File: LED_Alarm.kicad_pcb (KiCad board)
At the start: 2 copper layers, 48.3 x 82.8 mm, 84 parts, among them P101 CONN_01X06, Q301 Q_NPN_BCE, Q401 FDMA410NZT, Q402 FDMA410NZT, Q403 FDMA410NZT, Q501 FDMA410NZT, Q502 FDMA410NZT, Q503 FDMA410NZT, Q601 FDMA410NZT, Q602 FDMA410NZT, Q603 FDMA410NZT, Q701 FDMA410NZT, Q702 FDMA410NZT, Q703 FDMA410NZT, Q801 FDMA410NZT, Q802 FDMA410NZT, Q803 FDMA410NZT, U101 H11AA11, U102 ESP-12, U103 PCA9685PW, U201 MOC3020M, U202 TRIAC, U901 XC9263

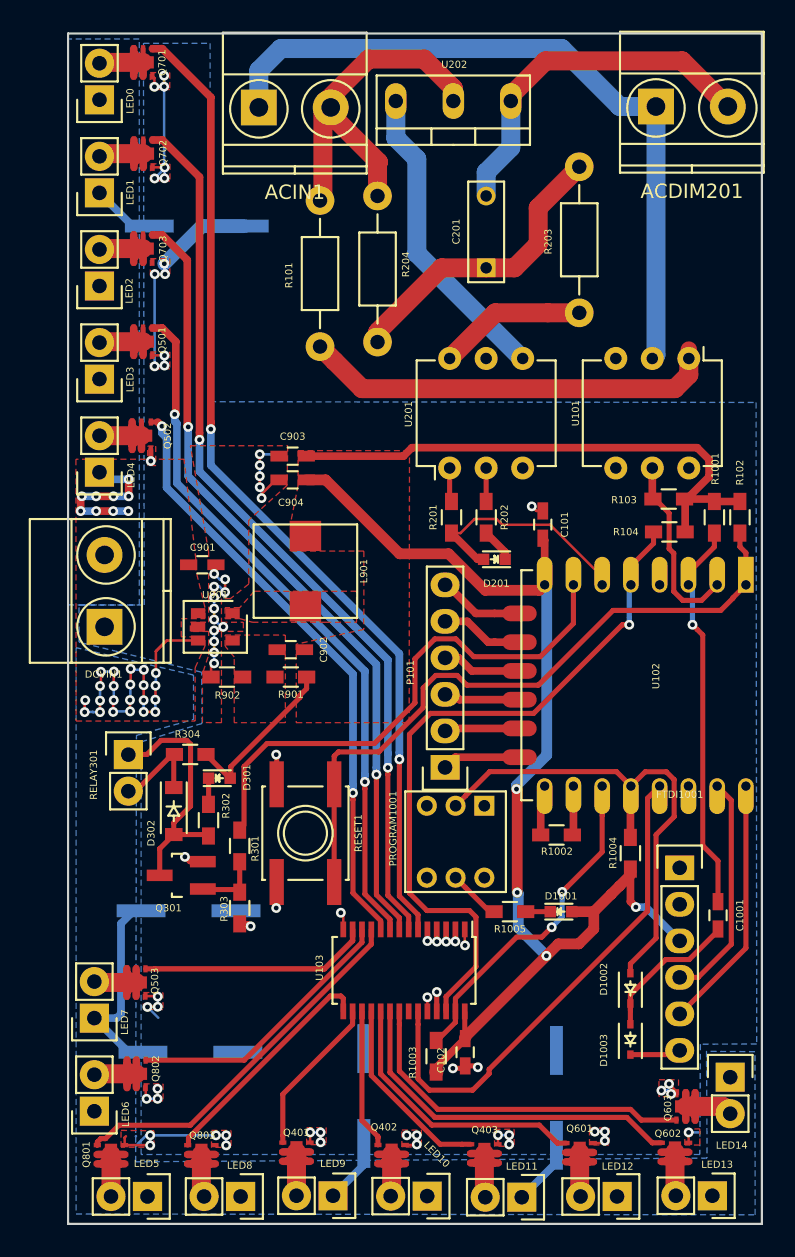
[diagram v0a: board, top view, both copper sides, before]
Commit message: changed some stuff around
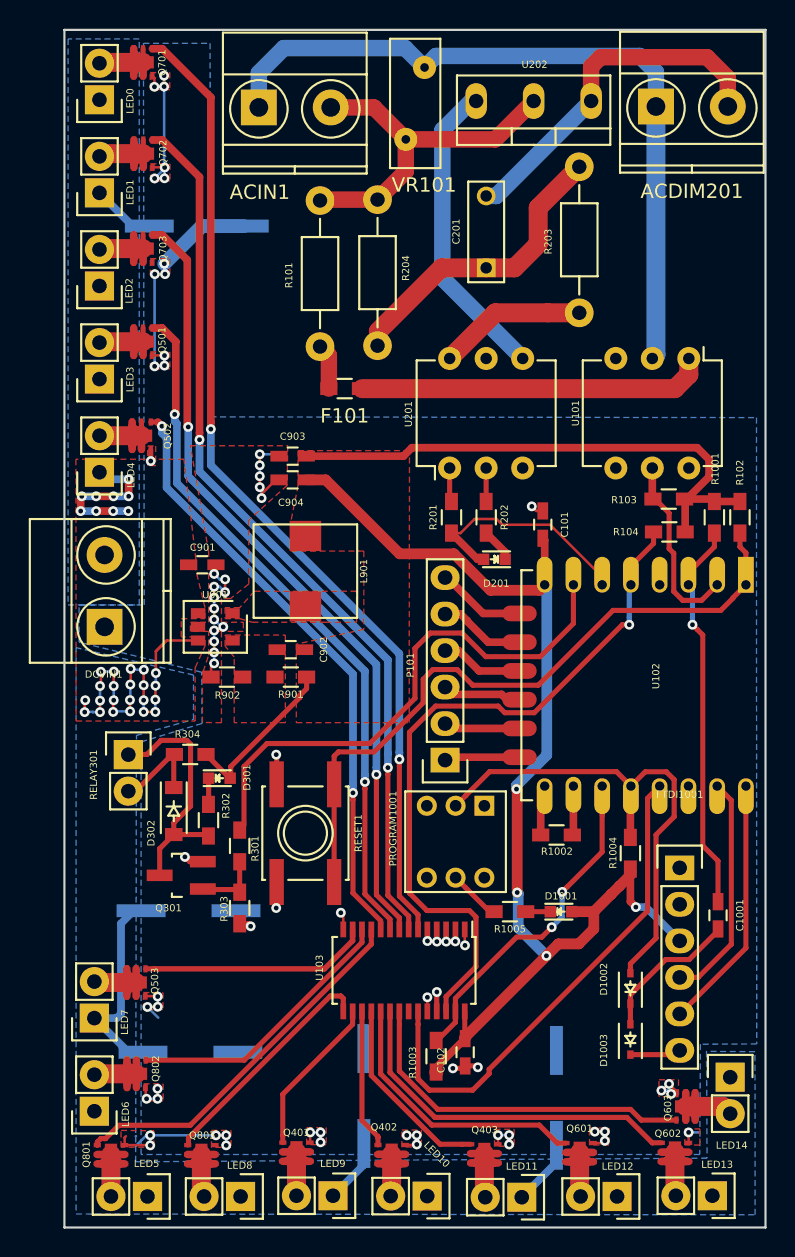
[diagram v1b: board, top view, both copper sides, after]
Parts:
- added F101: PRG18BB101MB1RB, Resistors_SMD:R_0603_HandSoldering, F.Cu at (71.3, 62.4)
- added VR101: MOV-07D221K-ND, Varistors:RV_Disc_D9_W3.5_P5, F.Cu at (75.6, 45.1)
- moved U202 5.59 mm to (84.5, 42.4)
- moved P101 0.51 mm to (78.3, 88.3)
- moved R204 0.25 mm to (73.6, 59.4)
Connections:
- R101 pad 2: Net-(R101-Pad2) -> Net-(F101-Pad2)
- U101 pad 1: Net-(R101-Pad2) -> Net-(F101-Pad1)
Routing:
- net Net-(R101-Pad2): track 29.0 -> 0.00 mm
- net Net-(F101-Pad1): track 0.00 -> 24.3 mm
- net Net-(F101-Pad2): track 0.00 -> 3.18 mm
- net GNDPWR: track 50.1 -> 52.1 mm
- net HT: track 26.4 -> 25.2 mm
- net Net-(C201-Pad1): track 21.0 -> 20.2 mm
- net /AC_CTRL2: track 36.6 -> 37.2 mm
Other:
- board size 48.3 x 82.8 mm -> 48.8 x 83.3 mm
- rule pad_to_mask_clearance: 0.1 -> 0.0762
